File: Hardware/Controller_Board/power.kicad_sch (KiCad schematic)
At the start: 54 parts, among them Q101 DMN2400UFB-7, U101 TPS82084, U102 LT8645S, U103 TDS5311P, U104 TPS82084, U105 TPS82084, U106 XT30

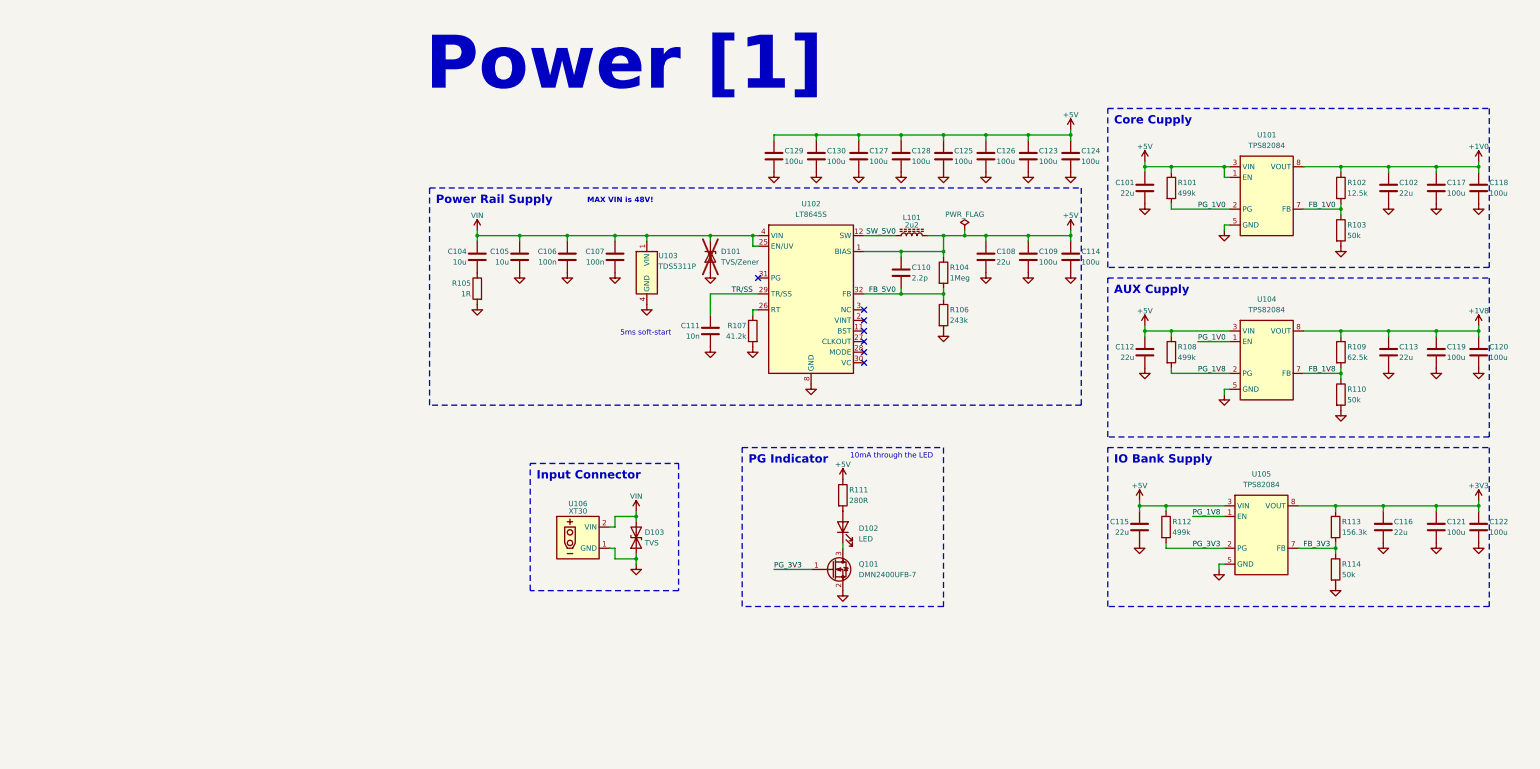
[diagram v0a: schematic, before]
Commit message: Advanced PCB Design: Routing Power + UVLO
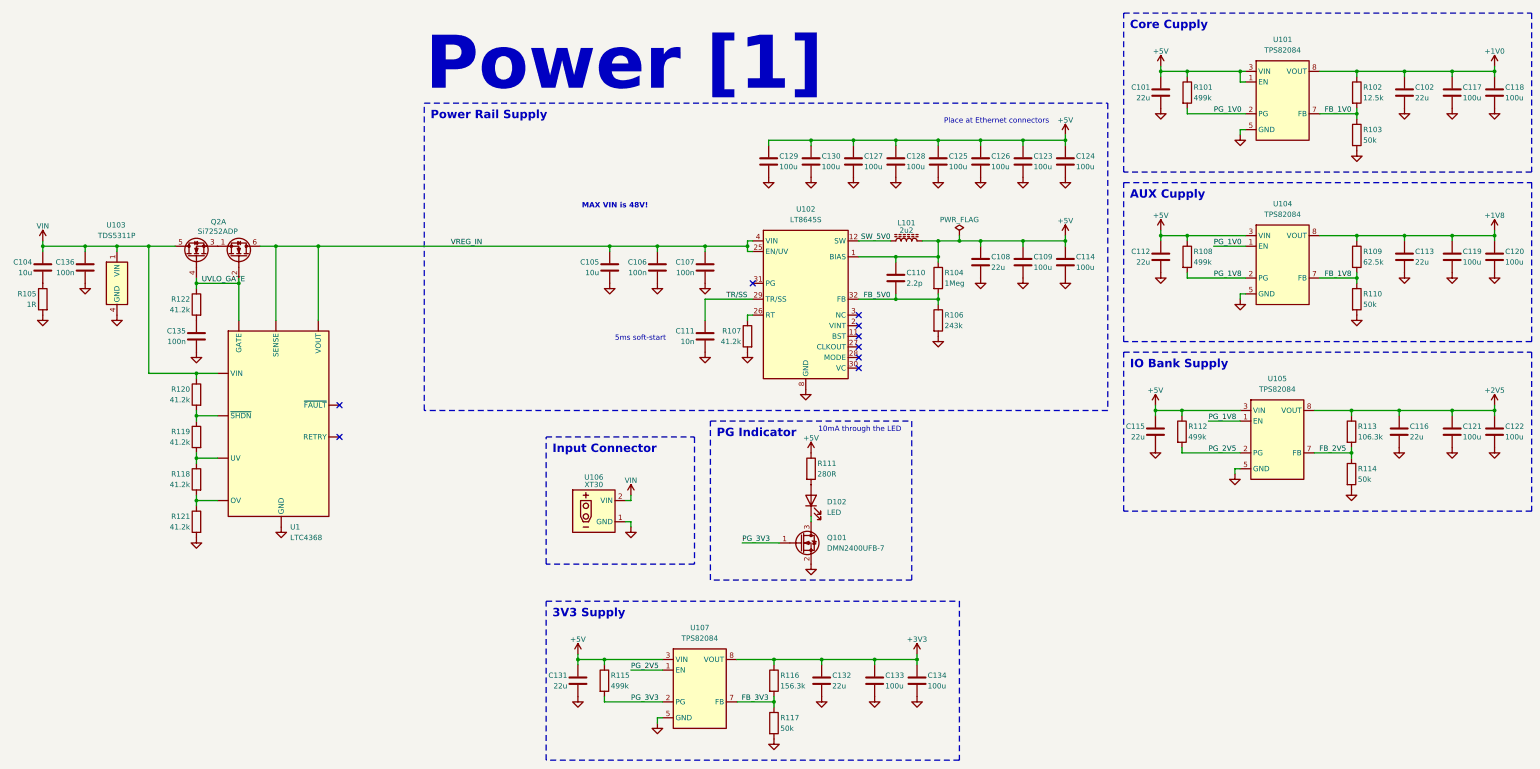
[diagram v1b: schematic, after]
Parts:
- removed D101: TVS/Zener, Diode_SMD:D_0603_1608Metric, symbol Device:D_Zener
- removed D103: TVS, Diode_SMD:D_0402_1005Metric, symbol Device:D_TVS
- added C131, C132: 22u, Capacitor_SMD:C_0603_1608Metric, symbol Device:C
- added C133, C134: 100u, Capacitor_SMD:C_1206_3216Metric, symbol Device:C
- added C135, C136: 100n, Capacitor_SMD:C_0805_2012Metric, symbol Device:C
- added Q2: Si7252ADP, Package_SO:PowerPAK_SO-8_Dual, symbol Transistor_FET:Q_Dual_NMOS_S1G1S2G2D2D1
- added R115: 499k, Resistor_SMD:R_0402_1005Metric, symbol Device:R
- added R116: 156.3k, Resistor_SMD:R_0402_1005Metric, symbol Device:R
- added R117: 50k, Resistor_SMD:R_0402_1005Metric, symbol Device:R
- added R118, R119, R120, R121, R122: 41.2k, Resistor_SMD:R_0402_1005Metric, symbol Device:R
- added U1: LTC4368, Package_DFN_QFN:DFN-10-1EP_3x3mm_P0.5mm_EP1.65x2.38mm, symbol Custom_VoxLink_Symbols:LTC4368
- added U107: TPS82084, Package_LGA:Texas_SIL0008C_MicroSiP-8-1EP_2.8x3mm_P0.65mm_EP1.1x1.9mm, symbol Custom_VoxLink_Symbols:TPS82084
- R113: value 156.3k -> 106.3k
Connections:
- net +3V3: now also C132.1, C133.1, C134.1, R116.1, U107.8 (VOUT); no longer C116.1, C121.1, C122.1, R113.1, U105.8 (VOUT)
- net +5V: now also C131.1, R115.1, U107.3 (VIN), U107.4 (VIN)
- net FB_3V3: now also R116.2, R117.1, U107.7 (FB); no longer R113.2, R114.1, U105.7 (FB)
- net GND: now also C131.2, C132.2, C133.2, C134.2, C135.2, C136.2, R117.2, R121.2, U1. (RETRY), U107.5 (GND), U107.6 (GND), U107.9 (GND)
- net PG_3V3: now also R115.2, U107.2 (PG); no longer R112.2, U105.2 (PG)
- net VIN: now also C136.1, Q2.5 (D), R120.1, U1. (RETRY); no longer C105.1, C106.1, C107.1, U102.21 (VIN), U102.22 (VIN), U102.23 (VIN), U102.25 (EN/UV), U102.4 (VIN), U102.5 (VIN), U102.6 (VIN)
- new net: R119.1, R120.2, U1. (RETRY)
- new net: R118.1, R119.2, U1. (RETRY)
- new net: R118.2, R121.1, U1. (RETRY)
- new net: C135.1, R122.2
- new net: Q2.1 (S), Q2.3 (S)
- new net +2V5: C116.1, C121.1, C122.1, R113.1, U105.8 (VOUT)
- new net FB_2V5: R113.2, R114.1, U105.7 (FB)
- new net PG_2V5: R112.2, U105.2 (PG), U107.1 (EN)
- new net UVLO_GATE: Q2.2 (G), Q2.4 (G), R122.1, U1. (RETRY)
- new net VREG_IN: C105.1, C106.1, C107.1, Q2.6 (D), U1. (RETRY), U102.21 (VIN), U102.22 (VIN), U102.23 (VIN), U102.25 (EN/UV), U102.4 (VIN), U102.5 (VIN), U102.6 (VIN)
- no-connect marks 7 -> 9
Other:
- note added: "Place at Ethernet connectors"
- moved on the sheet: C101, C102, C104, C105, C106, C107, C108, C109, C110, C111, C112, C113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

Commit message: Finished PCB Design - WARNING MORE CHANGES NEEDED! The main decision to be made is, whether to increase the layer count to 8 layers, and make the P7 and P8 permamently on 3V3
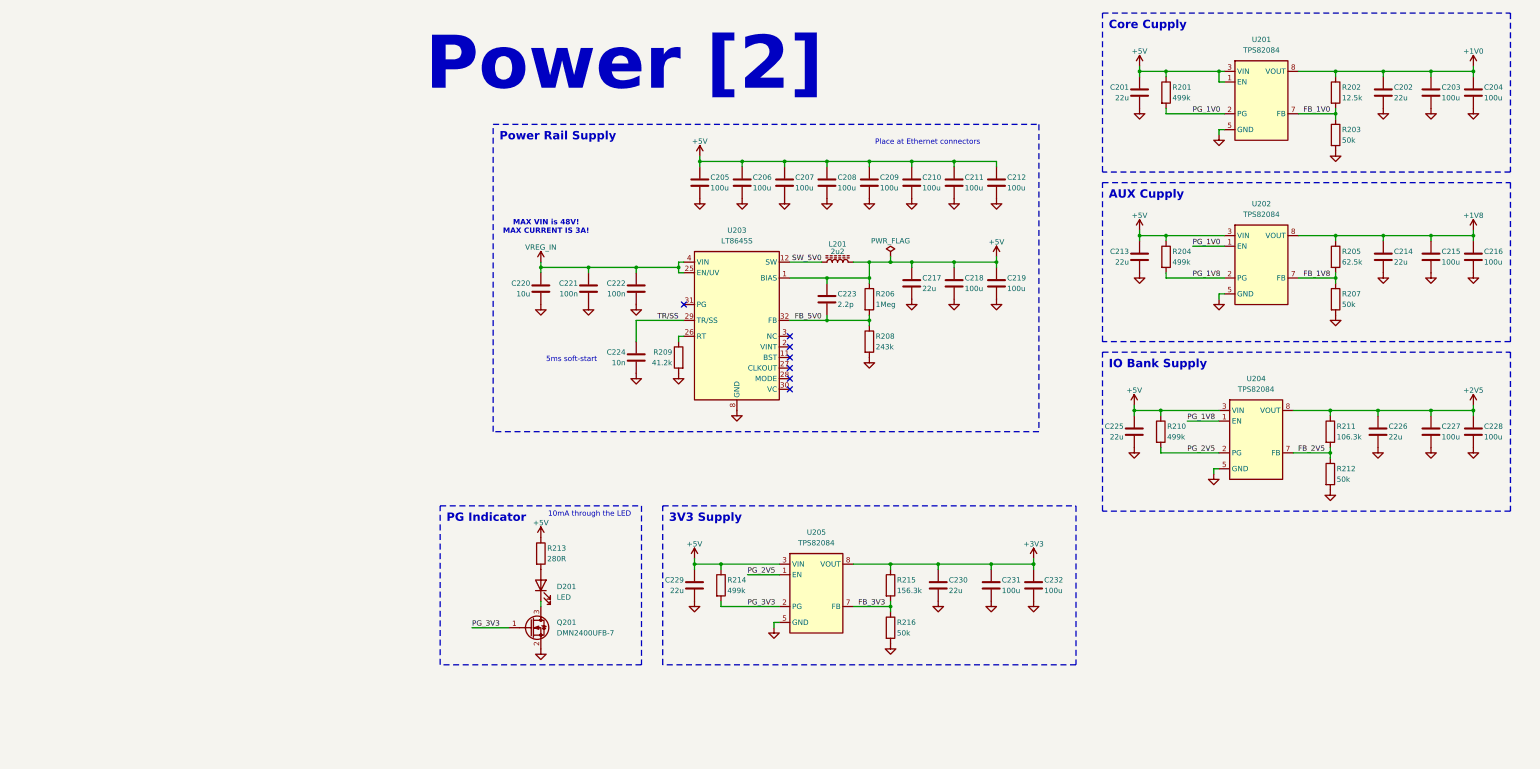
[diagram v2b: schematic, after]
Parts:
- removed C104: 10u, Capacitor_SMD:C_1206_3216Metric, symbol Device:C
- removed C135, C136: 100n, Capacitor_SMD:C_0805_2012Metric, symbol Device:C
- removed Q2: Si7252ADP, Package_SO:PowerPAK_SO-8_Dual, symbol Transistor_FET:Q_Dual_NMOS_S1G1S2G2D2D1
- removed R105: 1R, Resistor_SMD:R_0603_1608Metric, symbol Device:R
- removed R118, R119, R120, R121, R122: 41.2k, Resistor_SMD:R_0402_1005Metric, symbol Device:R
- removed U1: LTC4368, Package_DFN_QFN:DFN-10-1EP_3x3mm_P0.5mm_EP1.65x2.38mm, symbol Custom_VoxLink_Symbols:LTC4368
- removed U103: TDS5311P, Package_DFN_QFN:DFN-6-1EP_2x2mm_P0.65mm_EP1x1.6mm, symbol Custom_VoxLink_Symbols:TDS5311P
- removed U106: XT30, Connector_AMASS:AMASS_XT30PW-M_1x02_P2.50mm_Horizontal, symbol Custom_VoxLink_Symbols:Conn_XT
- renumbered C101 to C201, C102 to C202, C117 to C203, C118 to C204, C129 to C205, C130 to C206, C127 to C207, C128 to C208, C125 to C209, C126 to C210, C123 to C211, C124 to C212, C112 to C213, C113 to C214, C119 to C215, C120 to C216, C108 to C217, C109 to C218, C114 to C219, C105 to C220, C106 to C221, C107 to C222, C110 to C223, C111 to C224, C115 to C225, C116 to C226, C121 to C227, C122 to C228, C131 to C229, C132 to C230, C133 to C231, C134 to C232, D102 to D201, L101 to L201, Q101 to Q201, R101 to R201, R102 to R202, R103 to R203, R108 to R204, R109 to R205, R104 to R206, R110 to R207, R106 to R208, R107 to R209, R112 to R210, R113 to R211, R114 to R212, R111 to R213, R115 to R214, R116 to R215, R117 to R216, U101 to U201, U104 to U202, U102 to U203, U105 to U204, U107 to U205
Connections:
- no-connect marks 9 -> 7
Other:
- note added: "MAX VIN is 48V! MAX CURRENT IS 3A!"
- note added: "Power [2]"
- note removed: "MAX VIN is 48V!"
- note removed: "Power [1]"
- moved on the sheet: C201, C202, C203, C204, C205, C206, C207, C208, C209, C210, C211, C212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
